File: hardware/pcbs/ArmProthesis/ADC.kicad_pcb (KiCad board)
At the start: 4 copper layers, 60.3 x 44.8 mm, 27 parts, among them J1 H_16_2.54mm, SW1 SW_Reed_SPDT, SW2 SW_Reed_SPDT, SW3 SW_Reed_SPDT, SW4 SW_Reed_SPDT, U1 AD7606BSTZ

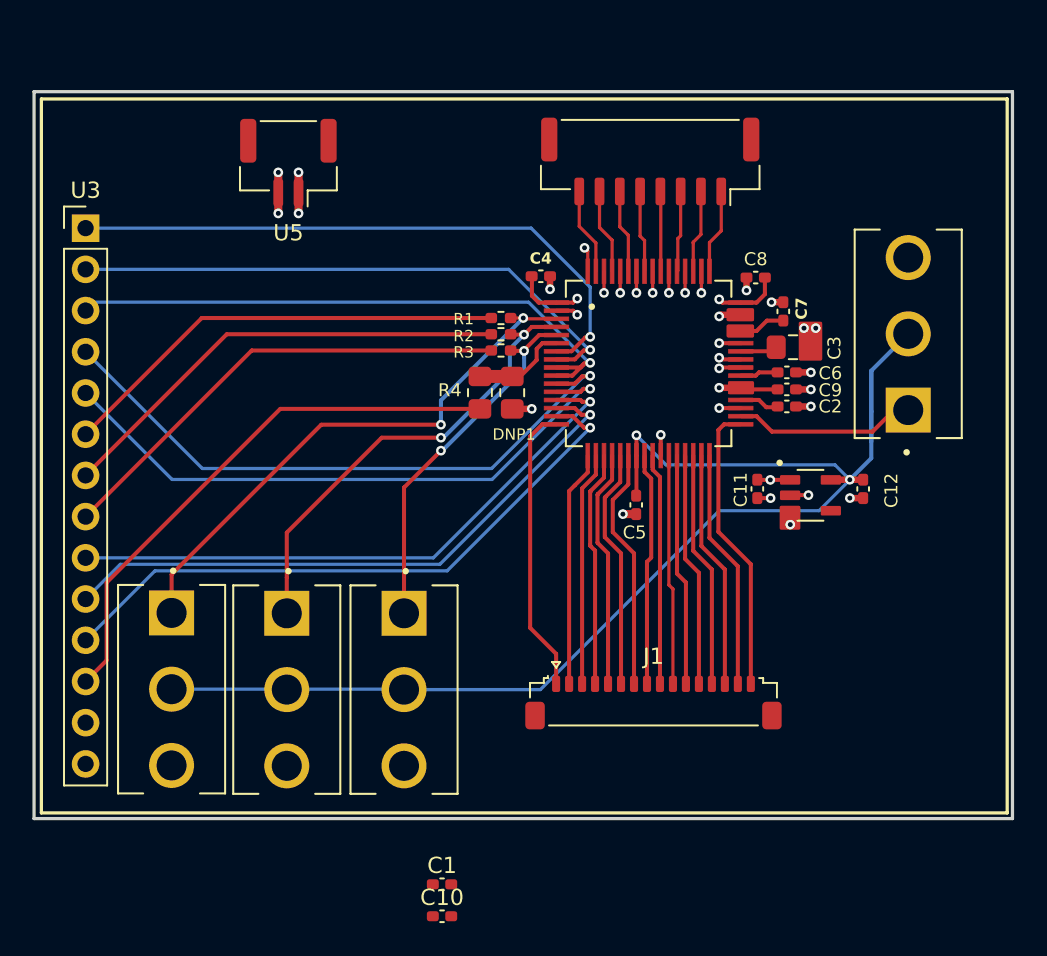
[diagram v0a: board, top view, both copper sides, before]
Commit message: BMS v0.3 + main folder reconstruction
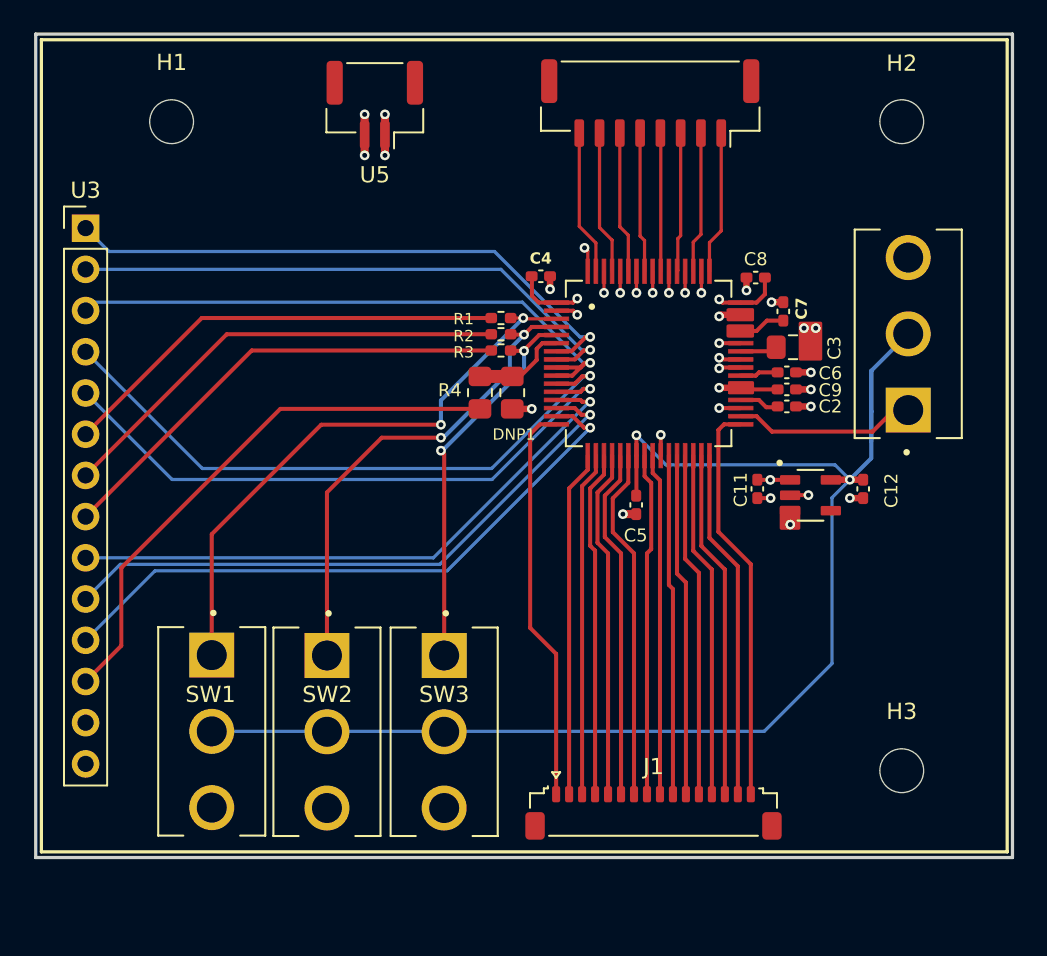
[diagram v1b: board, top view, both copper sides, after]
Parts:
- removed C1: 0.1uF, Capacitor_SMD:C_0402_1005Metric_Pad0.74x0.62mm_HandSolder
- removed C10: 1uF, Capacitor_SMD:C_0402_1005Metric_Pad0.74x0.62mm_HandSolder
- added H1: MountingHole, MountingHole:MountingHole_2.7mm_M2.5, F.Cu at (147.5, 70.0)
- added H2: MountingHole, MountingHole:MountingHole_2.7mm_M2.5, F.Cu at (192.5, 70.0)
- added H3: MountingHole, MountingHole:MountingHole_2.7mm_M2.5, F.Cu at (192.5, 110.0)
- moved J1 6.80 mm to (177.2, 112.6)
- moved U5 6.41 mm to (160.0, 69.0)
- moved U2 3.60 mm to (177.0, 68.8)
- moved SW3 3.59 mm to (164.3, 107.6)
- moved SW1 3.59 mm to (150.0, 107.6)
- moved SW2 3.59 mm to (157.1, 107.6)
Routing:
- net DB0: track 17.8 -> 24.7 mm
- net DB8DOUTB: track 14.3 -> 21.1 mm
- net DB4: track 14.7 -> 21.5 mm
- net DB1: track 14.5 -> 21.3 mm
- net DB13: track 14.7 -> 21.5 mm
- net DB11: track 14.4 -> 21.2 mm
- net DB10: track 14.3 -> 21.1 mm
- net DB9: track 14.2 -> 21.0 mm
- net DB6: track 15.0 -> 21.8 mm
- net DB7/DOUTA: track 14.3 -> 21.1 mm
- net DB14: track 14.8 -> 21.6 mm
- net DB12: track 14.5 -> 21.3 mm
- net DB5: track 14.9 -> 21.7 mm
- net DB3: track 14.5 -> 21.3 mm
- net DB15: track 18.0 -> 24.8 mm
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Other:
- board size 60.3 x 44.8 mm -> 60.2 x 50.8 mm

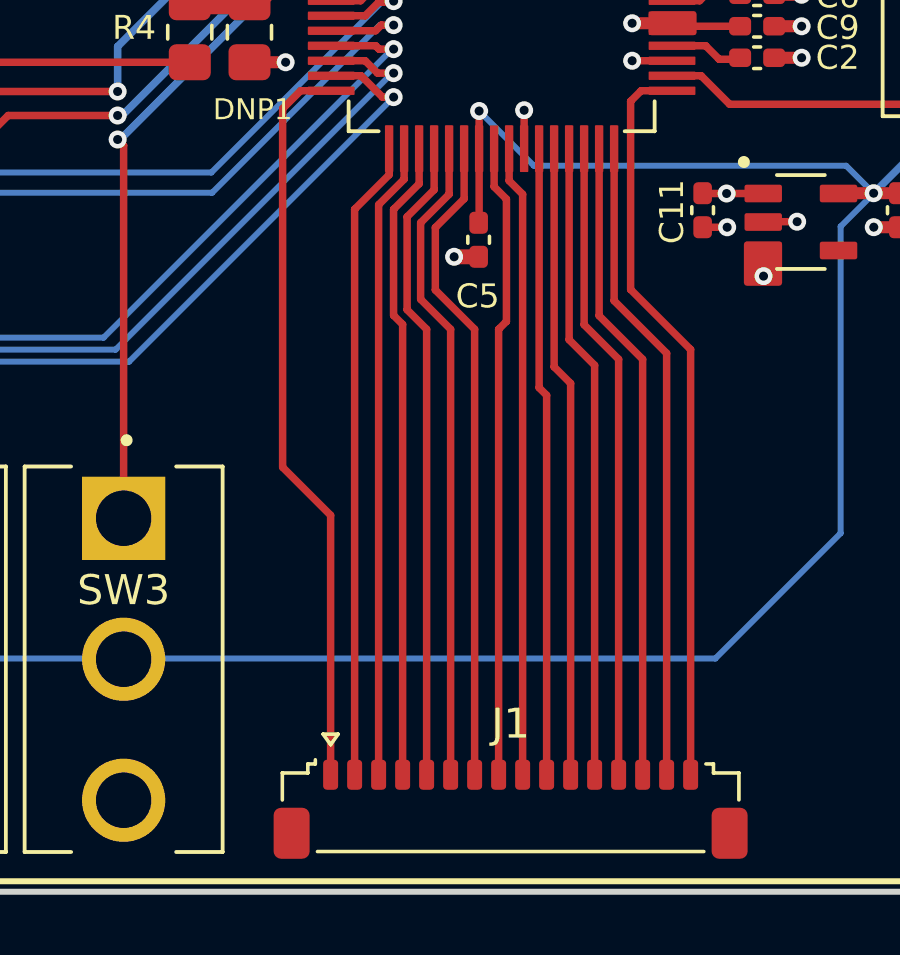
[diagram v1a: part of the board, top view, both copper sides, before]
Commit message: .
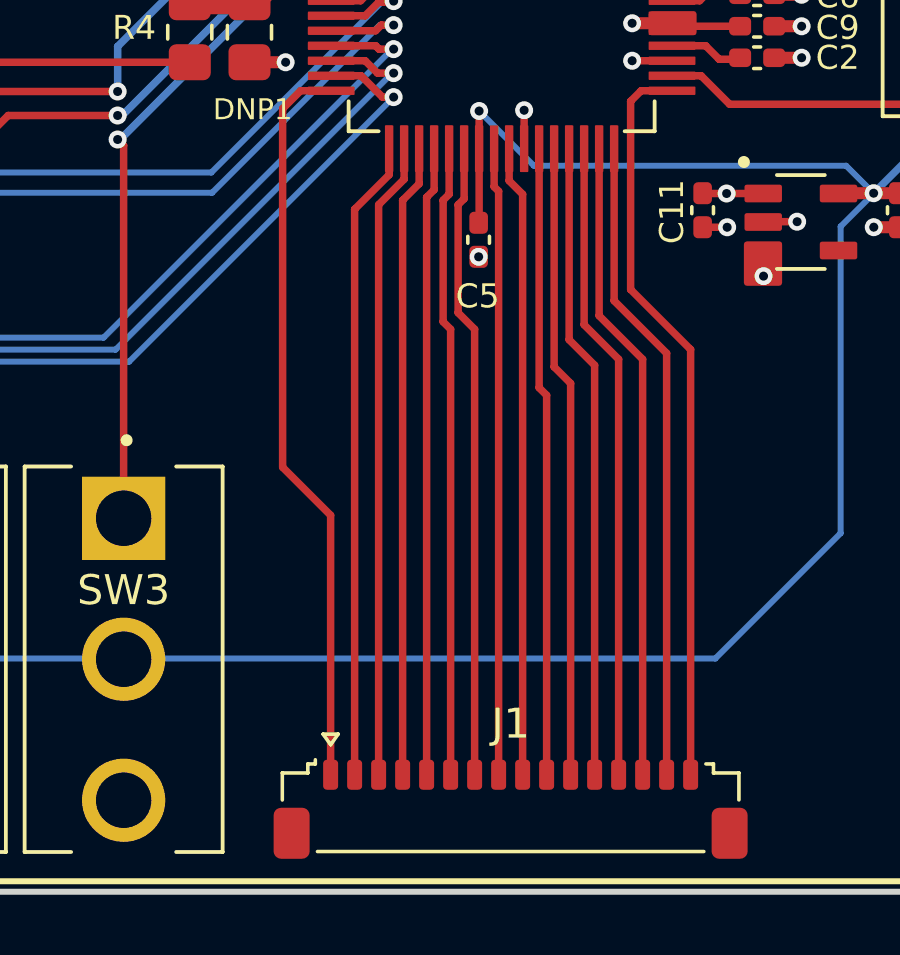
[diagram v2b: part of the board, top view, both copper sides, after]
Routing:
- net GND: track 32.4 -> 31.6 mm
- net DB6: track 21.8 -> 21.2 mm
- net DB5: track 21.7 -> 21.1 mm
- net DB4: track 21.5 -> 21.0 mm
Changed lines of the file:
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@@
-	)
-	(segment
-		(start 176.13375 94.185)
-		(end 175.31625 94.185)
-		(width 0.5)
-		(layer "F.Cu")
-		(net 1)
 	)
 	(segment
@@
 	)
 	(via
-		(at 175.31625 94.185)
+		(at 176.13375 94.185)
 		(size 0.6)
 		(drill 0.3)
@@
 	(segment
 		(start 175.65 92.25)
-		(end 174.69025 93.20975)
-		(width 0.25)
-		(layer "F.Cu")
-		(net 19)
-	)
-	(segment
-		(start 174.69025 93.20975)
-		(end 174.69025 95.29025)
+		(end 175.45 92.45)
 		(width 0.25)
 		(layer "F.Cu")
@@
 	)
 	(segment
+		(start 175.45 92.45)
+		(end 175.45 96.05)
+		(width 0.25)
+		(layer "F.Cu")
+		(net 19)
+	)
+	(segment
+		(start 175.45 96.05)
+		(end 176 96.6)
+		(width 0.25)
+		(layer "F.Cu")
+		(net 19)
+	)
+	(segment
 		(start 175.65 90.58)
 		(end 175.65 92.25)
@@
 	)
 	(segment
-		(start 174.69025 95.29025)
-		(end 176 96.6)
-		(width 0.25)
-		(layer "F.Cu")
-		(net 19)
-	)
-	(segment
 		(start 181.2 89)
 		(end 181.2 95.275)
@@
 	)
 	(segment
-		(start 174.15 91.75)
-		(end 173.298 92.602)
-		(width 0.25)
-		(layer "F.Cu")
-		(net 30)
-	)
-	(segment
-		(start 173.298 92.602)
-		(end 173.298 96.13581)
-		(width 0.25)
-		(layer "F.Cu")
-		(net 30)
-	)
-	(segment
-		(start 173.6 96.43781)
-		(end 173.6 111.45)
-		(width 0.25)
-		(layer "F.Cu")
-		(net 30)
-	)
-	(segment
-		(start 173.298 96.13581)
-		(end 173.6 96.43781)
-		(width 0.25)
-		(layer "F.Cu")
-		(net 30)
-	)
-	(segment
 		(start 174.15 90.58)
 		(end 174.15 91.75)
@@
 	)
 	(segment
+		(start 173.6 92.3)
+		(end 173.6 111.45)
+		(width 0.25)
+		(layer "F.Cu")
+		(net 30)
+	)
+	(segment
+		(start 174.15 91.75)
+		(end 173.6 92.3)
+		(width 0.25)
+		(layer "F.Cu")
+		(net 30)
+	)
+	(segment
 		(start 176.65 77.325)
 		(end 176.375 77.05)
@@
 	)
 	(segment
-		(start 176.8 96.6)
+		(start 176.65 91.85)
+		(end 176.8 92)
+		(width 0.25)
+		(layer "F.Cu")
+		(net 33)
+	)
+	(segment
+		(start 176.8 92)
 		(end 176.8 111.45)
-		(width 0.25)
-		(layer "F.Cu")
-		(net 33)
-	)
-	(segment
-		(start 177.06 96.34)
-		(end 176.8 96.6)
 		(width 0.25)
 		(layer "F.Cu")
@@
 	)
 	(segment
-		(start 177.06 92.26)
-		(end 177.06 96.34)
-		(width 0.25)
-		(layer "F.Cu")
-		(net 33)
-	)
-	(segment
-		(start 176.65 91.85)
-		(end 177.06 92.26)
-		(width 0.25)
-		(layer "F.Cu")
-		(net 33)
-	)
-	(segment
 		(start 181.6 97.6)
 		(end 181.6 111.45)
@@
 	)
 	(segment
-		(start 173.749 95.949)
-		(end 174.4 96.6)
-		(width 0.25)
-		(layer "F.Cu")
-		(net 37)
-	)
-	(segment
-		(start 174.4 96.6)
-		(end 174.4 111.45)
-		(width 0.25)
-		(layer "F.Cu")
-		(net 37)
-	)
-	(segment
 		(start 174.65 91.95)
-		(end 173.749 92.851)
+		(end 174.4 92.2)
 		(width 0.25)
 		(layer "F.Cu")
@@
 	)
 	(segment
-		(start 173.749 92.851)
-		(end 173.749 95.949)
+		(start 174.4 92.2)
+		(end 174.4 111.45)
 		(width 0.25)
 		(layer "F.Cu")
@@
 	)
 	(segment
-		(start 175.15 92.1)
-		(end 174.2 93.05)
+		(start 174.95 92.3)
+		(end 174.95 96.35)
 		(width 0.25)
 		(layer "F.Cu")
@@
 	)
 	(segment
-		(start 174.2 93.05)
-		(end 174.2 95.6)
-		(width 0.25)
-		(layer "F.Cu")
-		(net 42)
-	)
-	(segment
-		(start 174.2 95.6)
-		(end 175.2 96.6)
+		(start 175.15 92.1)
+		(end 174.95 92.3)
 		(width 0.25)
 		(layer "F.Cu")
@@
 		(width 0.25)
 		(layer "F.Cu")
+		(net 42)
+	)
+	(segment
+		(start 174.95 96.35)
+		(end 175.2 96.6)
+		(width 0.25)
+		(layer "F.Cu")
